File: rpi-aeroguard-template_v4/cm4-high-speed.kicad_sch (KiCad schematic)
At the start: 2 parts, among them J1 F305-1A7H1-21022-E100, J7 DF40C-100DS-0.4V_51_

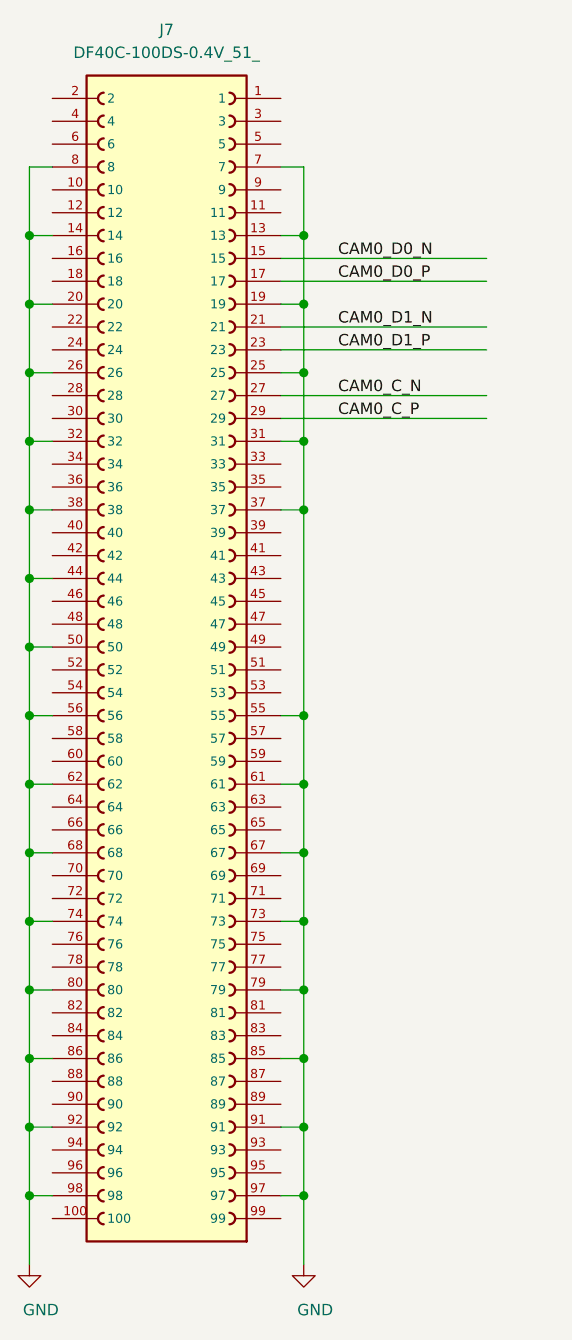
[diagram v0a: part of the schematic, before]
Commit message: Add files via upload
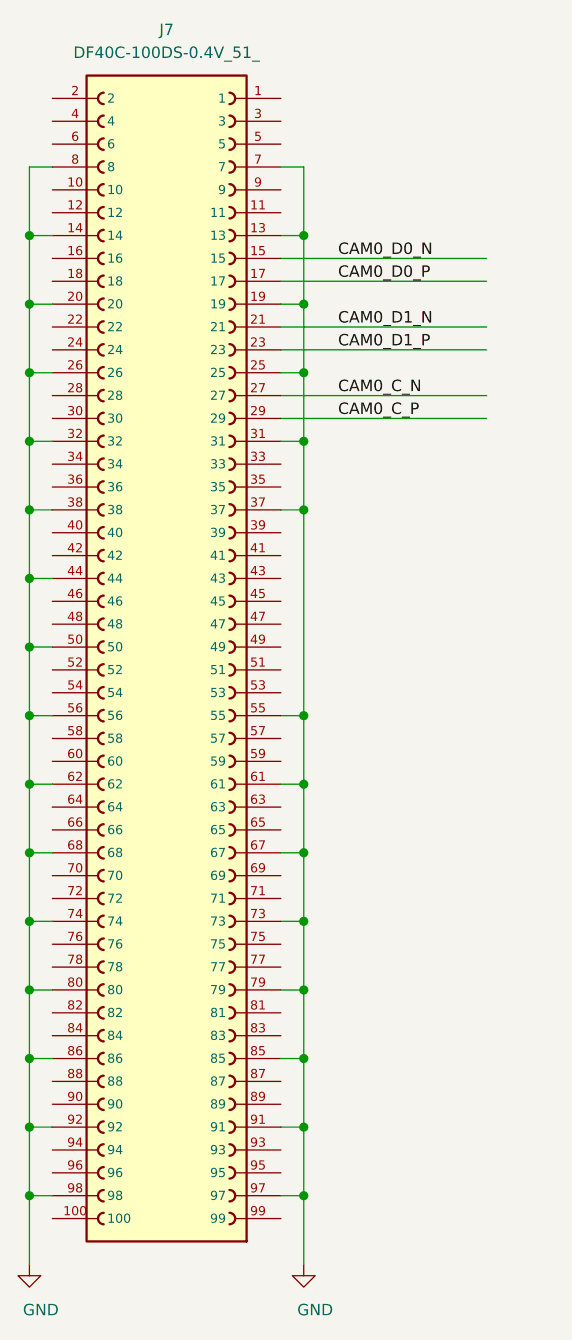
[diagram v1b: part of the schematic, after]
